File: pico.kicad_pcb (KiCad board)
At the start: 2 copper layers, 103 x 101.2 mm, 112 parts, among them J101 Conn_01x03, J103 XT60, J104 Conn_01x03, J105 Conn_01x03, J106 Conn_01x03, J107 Conn_01x03, J108 Conn_01x03, Q101 AGM30P100D, Q102 BSS138, Q103 AGM30P100D, Q104 AGM30P100D, Q105 AGM30P100D, Q106 AGM30P100D, Q201 SQJ142EP-T1_GE3, Q202 SQJ142EP-T1_GE3, Q203 SQJ142EP-T1_GE3, Q204 SQJ142EP-T1_GE3, Q205 SQJ142EP-T1_GE3, Q206 SQJ142EP-T1_GE3, Q301 SQJ142EP-T1_GE3, Q302 SQJ142EP-T1_GE3, Q303 SQJ142EP-T1_GE3, Q304 SQJ142EP-T1_GE3, Q305 SQJ142EP-T1_GE3, Q306 SQJ142EP-T1_GE3, U101 TPS7A2033PDBVR, U106 ADC124S051CIMM/NOPB, U201 DRV8323SRTAT, U301 DRV8323SRTAT

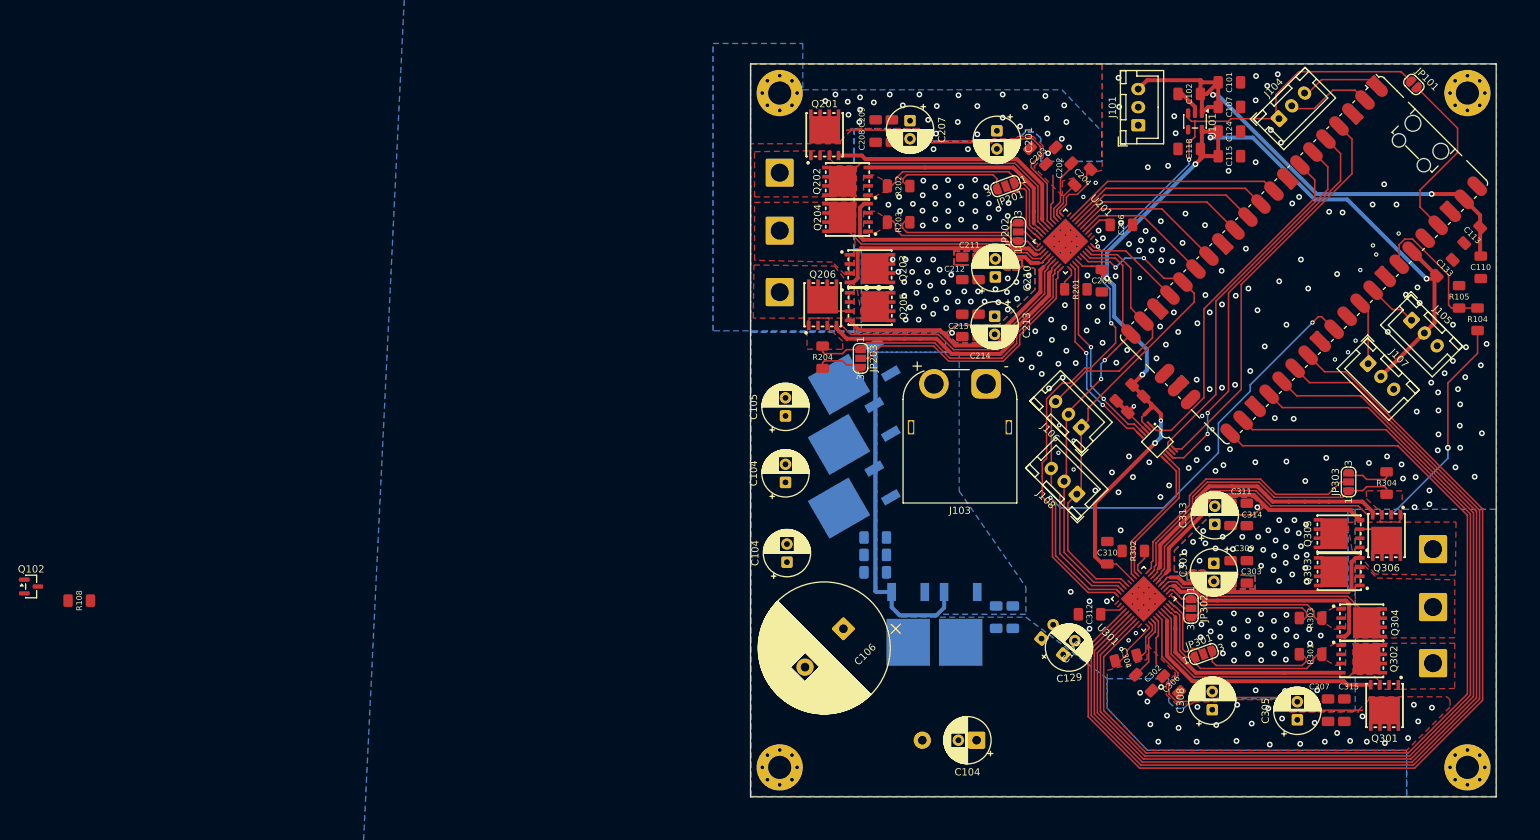
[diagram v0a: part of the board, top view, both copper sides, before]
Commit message: m, mn,
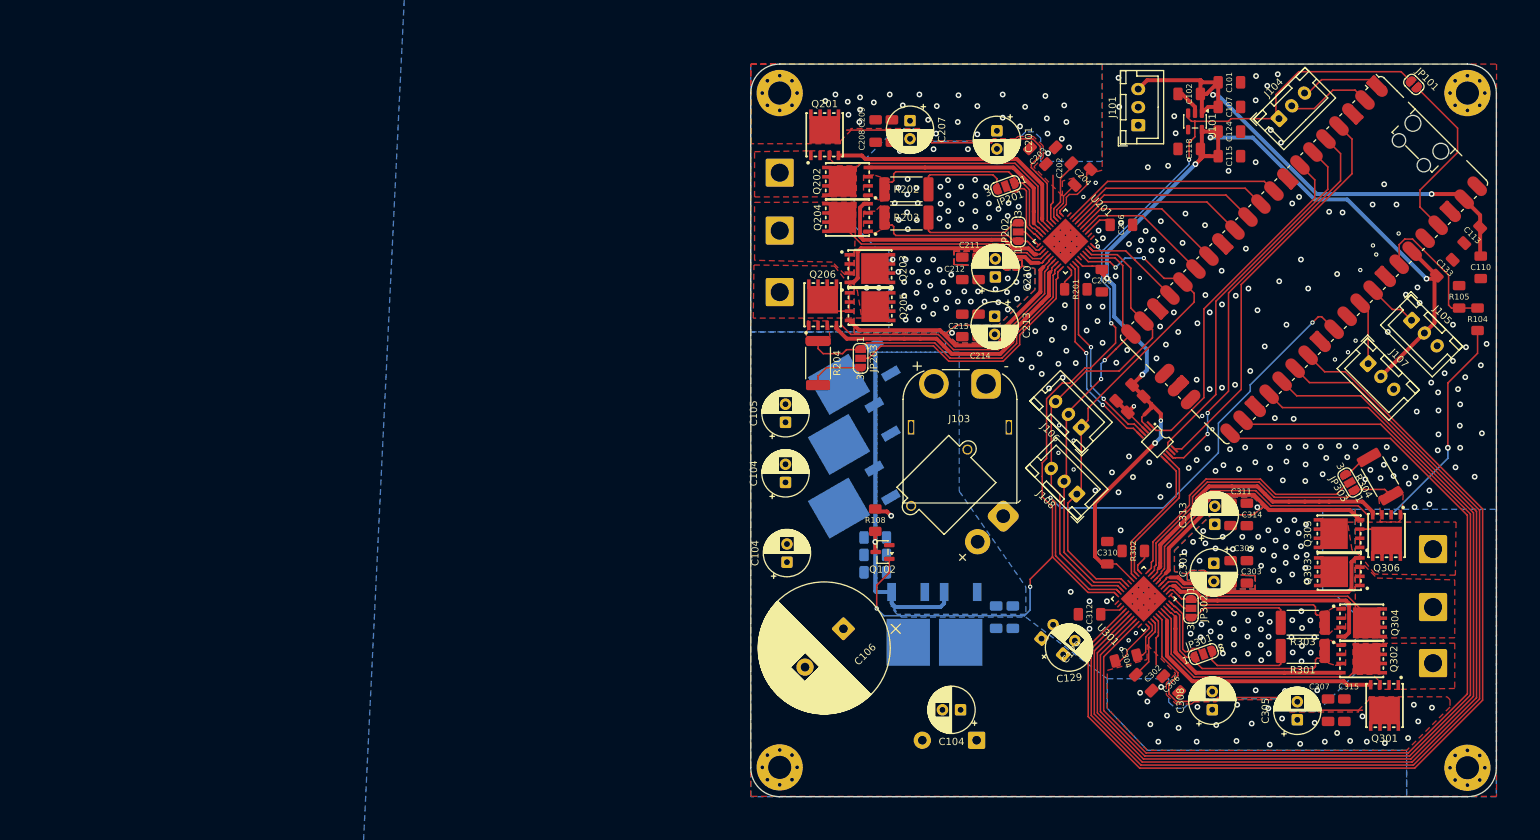
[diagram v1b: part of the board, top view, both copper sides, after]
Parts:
- added REF**: AMASS_XT30PW-M_1x02_P2.50mm_Horizontal, Connector_AMASS:AMASS_XT30PW-M_1x02_P2.50mm_Horizontal, F.Cu at (45.4, 122.7)
- R202, R203, R204, R301, R303, R304: footprint COMPONENTS:1206_Resistor -> Resistor_SMD:R_2512_6332Metric_Pad1.40x3.35mm_HandSolder
- moved Q102 117.7 mm to (28.7, 127.7), turned to 180 degrees
- moved R108 110.5 mm to (27.7, 123.3), turned to -90 degrees
- moved C104 4.74 mm to (39.5, 149.5)
- moved R304 1.27 mm to (97.5, 117.3), turned to 120 degrees
- moved R203 1.25 mm to (32.0, 81.5)
- moved R303 1.25 mm to (86.8, 137.5)
- moved R202 1.17 mm to (32.0, 77.6)
- moved R301 1.16 mm to (86.8, 141.3)
- moved R204 1.02 mm to (19.8, 101.6)
- moved C105 0.88 mm to (15.3, 109.8)
- moved JP303 0.19 mm to (93.3, 118.1), turned to 120 degrees
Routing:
- net ENable: track 123.8 -> 161.2 mm, vias 3 -> 5
- net GND: track 94.9 -> 78.1 mm, vias 231 -> 257
- net /IN: track 0.00 -> 2.59 mm, vias 0 -> 1
- net Net-(U201-CPH): track 8.02 -> 5.59 mm
- net Net-(Q101-G): track 49.0 -> 50.3 mm, vias 0 -> 1
- net /MotorDriver/Z_S_H: track 43.2 -> 44.3 mm
- net /MotorDriver/X_S_H: track 29.2 -> 29.8 mm
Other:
- outline, holes or cut-outs redrawn
- board text added: "3"
